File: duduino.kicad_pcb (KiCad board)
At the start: 2 copper layers, 64 x 42 mm, 20 parts, among them J1 USB_B, J2 FTDI, J3 IIC, J4 AVRKit, SW1 RESET, U1 LM3940, U2 ATMEGA168-20PU, Y1 Crystal

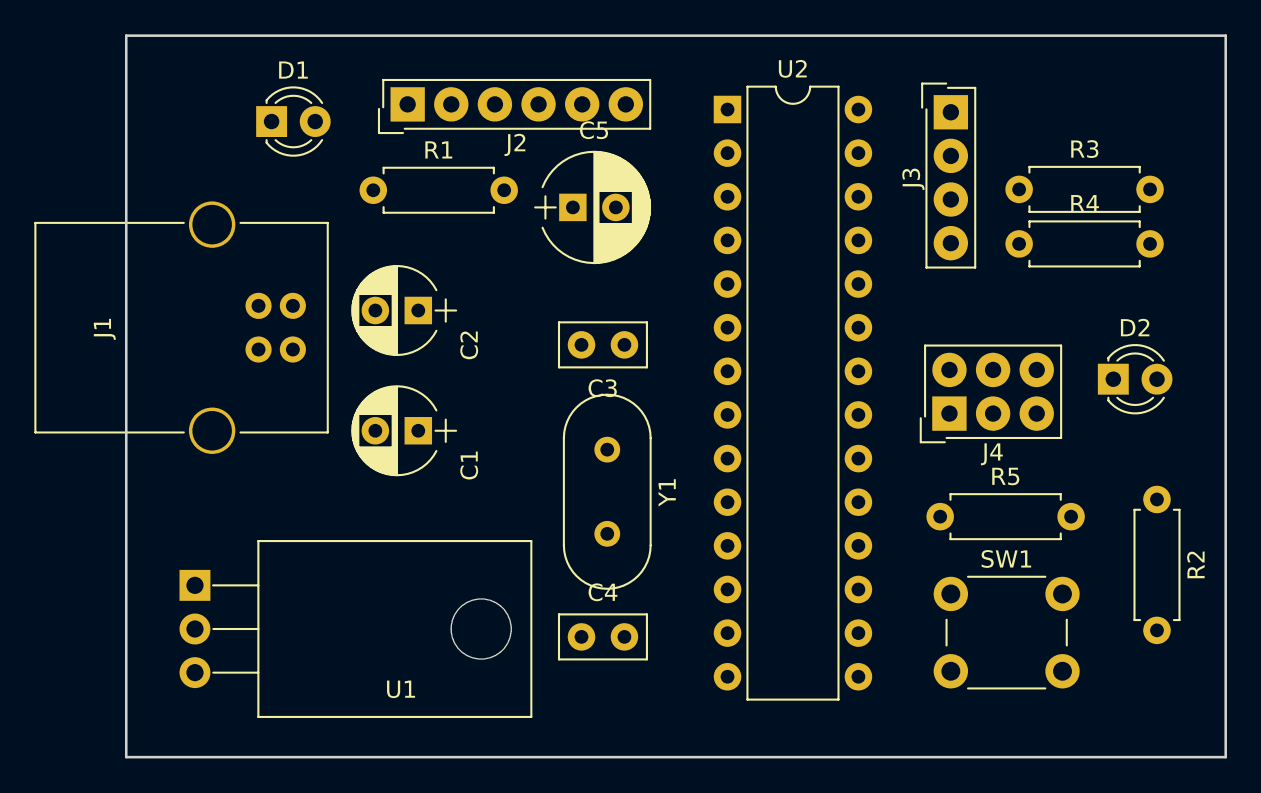
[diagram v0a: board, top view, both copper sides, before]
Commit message: tweaking the layout, upgrading Kicad, crying a little bit, then wiring all the PCB
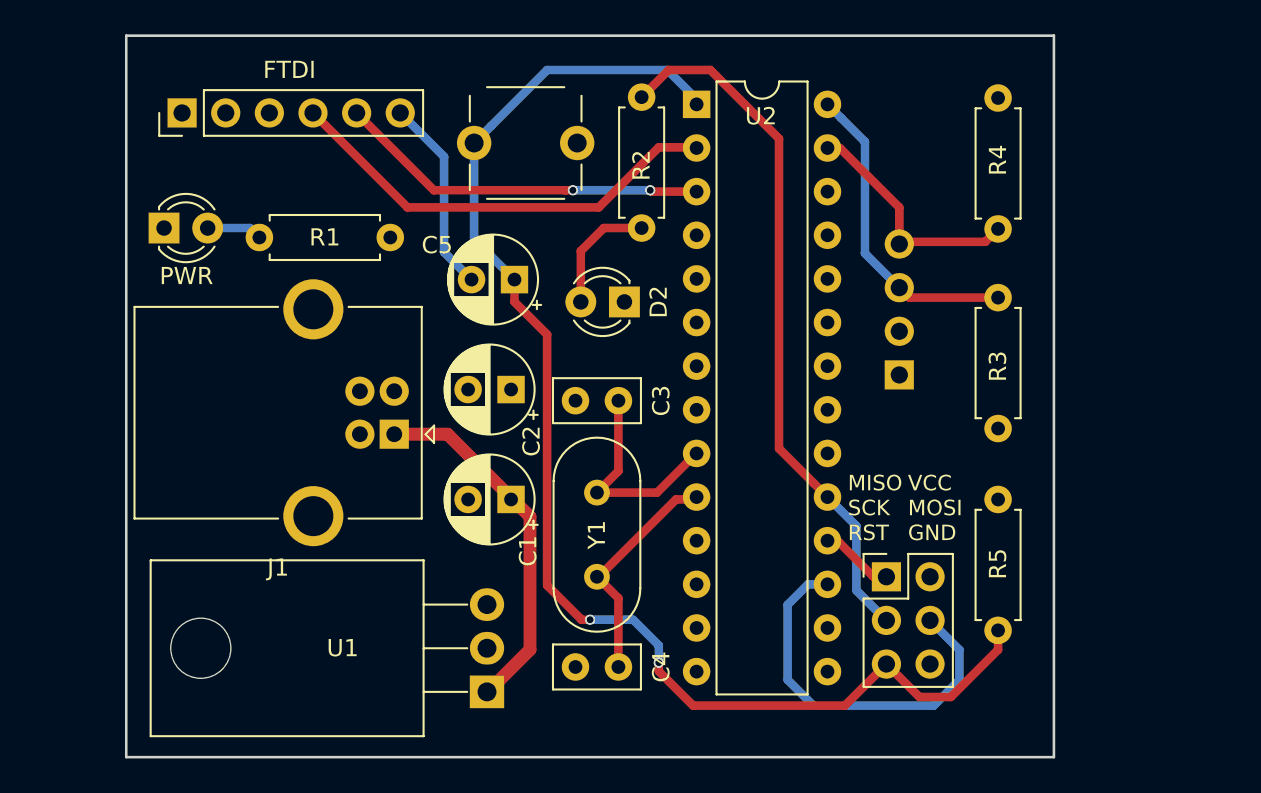
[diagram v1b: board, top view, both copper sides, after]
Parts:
- C1, C2: footprint Capacitors_THT:CP_Radial_D5.0mm_P2.50mm -> Capacitor_THT:CP_Radial_D5.0mm_P2.50mm
- C5: footprint Capacitors_THT:CP_Radial_D6.3mm_P2.50mm -> Capacitor_THT:CP_Radial_D5.0mm_P2.50mm
- J1: footprint Connectors:USB_B -> Connector_USB:USB_B_OST_USB-B1HSxx_Horizontal
- J2: footprint Connectors_Samtec:SL-106-X-XX_1x06 -> Connector_PinHeader_2.54mm:PinHeader_1x06_P2.54mm_Vertical
- J3: footprint Connectors_Samtec:SL-104-X-XX_1x04 -> duduino:SPI-OLED; moved to B.Cu
- J4: footprint Connectors_Samtec:SDL-106-X-XX_2x03 -> Connector_PinHeader_2.54mm:PinHeader_2x03_P2.54mm_Vertical
- SW1: footprint Buttons_Switches_THT:SW_PUSH_6mm_h5mm -> duduino:SW_PUSH_6mm
- U1: value LM3940 -> LM3940_TO220; footprint TO_SOT_Packages_THT:TO-220-3_Horizontal -> Package_TO_SOT_THT:TO-220-3_Horizontal_TabDown
- moved SW1 40.0 mm to (130.0, 112.0)
- moved R2 33.9 mm to (140.0, 119.2), turned to 90 degrees
- moved D2 28.8 mm to (139.0, 123.5), turned to 180 degrees
- moved U1 18.1 mm to (131.0, 146.2), turned to 90 degrees
- moved J3 15.6 mm to (155.0, 127.8)
- moved J2 13.1 mm to (113.2, 112.5)
- moved J4 10.2 mm to (154.2, 139.5), turned to 0 degrees
- moved D1 8.81 mm to (112.2, 119.2)
- moved J1 7.69 mm to (125.6, 131.2)
- moved R1 7.18 mm to (117.8, 119.8)
- moved C2 7.09 mm to (132.4, 128.6)
- moved C1 6.72 mm to (132.4, 135.0)
- moved R3 6.42 mm to (160.8, 123.2), turned to 270 degrees
- moved C5 5.40 mm to (132.6, 122.2), turned to 180 degrees
- moved R5 3.52 mm to (160.8, 135.0), turned to 270 degrees
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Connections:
- J2 pad 2: GND -> Net-(J2-Pad2)
- J2 pad 4: /TXD -> /RXD
- J2 pad 5: /RXD -> /TXD
- J3 pad 1: +3V3 -> GND
- J3 pad 2: GND -> +3V3
- J4 pad 2: /SCK -> +3V3
- J4 pad 3: /RST -> /SCK
- J4 pad 4: +3V3 -> /MOSI
- J4 pad 5: /MOSI -> /RST
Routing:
- net /RST: track 0.00 -> 77.3 mm, vias 0 -> 2
- net /SCK: track 0.00 -> 40.9 mm
- net /RXD: track 0.00 -> 26.1 mm
- net /MOSI: track 0.00 -> 22.6 mm
- net /TXD: track 0.00 -> 21.7 mm, vias 0 -> 2
- net +5V: track 0.00 -> 21.2 mm
- net /I2C_SCL: track 0.00 -> 18.4 mm
- net /I2C_SDA: track 0.00 -> 13.9 mm
- net /XTAL2: track 0.00 -> 13.5 mm
- net /XTAL1: track 0.00 -> 12.6 mm
- net /DTR: track 0.00 -> 11.4 mm
- net Net-(D2-Pad2): track 0.00 -> 7.06 mm
- net /MISO: track 0.00 -> 4.30 mm
- net Net-(D1-Pad2): track 0.00 -> 3.24 mm
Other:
- board size 64 x 42 mm -> 54 x 42 mm
- net class Default: trace_width 0.25 -> 0.5
- board text added: "GND CTS VCC RXD TXD DTR"
- board text added: "MISO SCK RST"
- board text added: "SDA SCL VCC GND"
- board text added: "VCC MOSI GND"
